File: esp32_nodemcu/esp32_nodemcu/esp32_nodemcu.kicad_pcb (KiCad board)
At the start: 2 copper layers, 17.8 x 30.5 mm, 3 parts, among them J1 Conn_01x02_Female

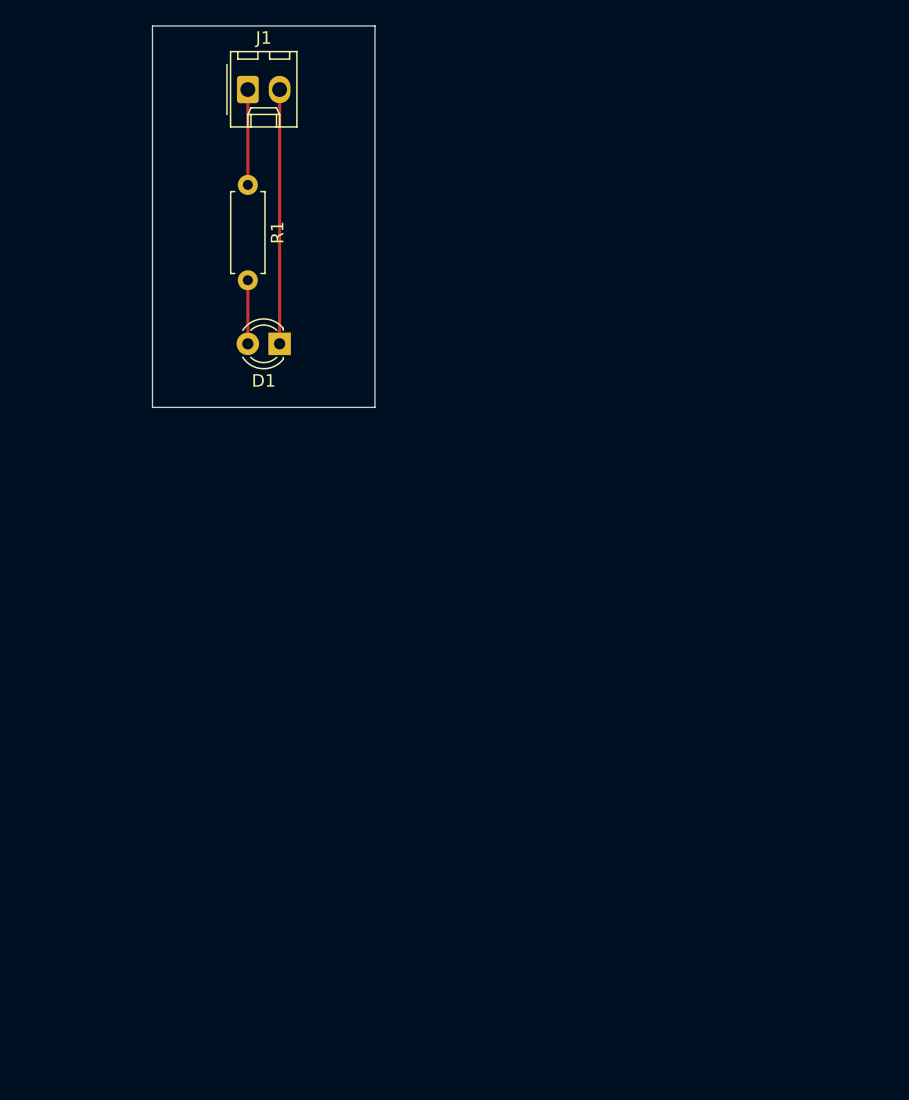
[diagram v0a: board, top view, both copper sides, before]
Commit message: pcb update
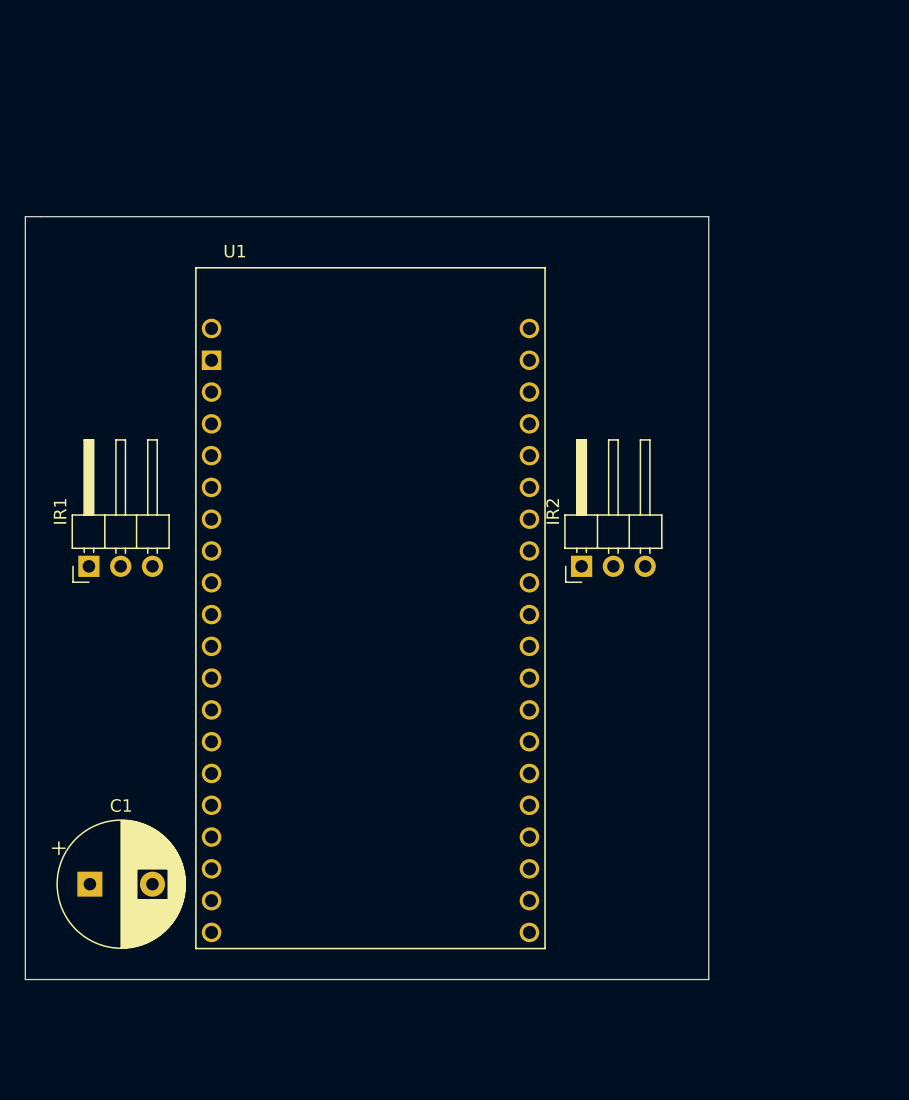
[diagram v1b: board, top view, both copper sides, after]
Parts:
- removed D1: LED, LED_THT:LED_D3.0mm
- removed J1: Conn_01x02_Female, Connector_Molex:Molex_KK-254_AE-6410-02A_1x02_P2.54mm_Vertical
- removed R1: R, Resistor_THT:R_Axial_DIN0207_L6.3mm_D2.5mm_P7.62mm_Horizontal
- added C1: CAP, Capacitor_THT:CP_Radial_D10.0mm_P5.00mm, F.Cu at (127.1, 124.5)
- added IR1: szh-ssbh-002, Connector_PinHeader_2.54mm:PinHeader_1x03_P2.54mm_Horizontal, F.Cu at (127.0, 99.1)
- added IR2: szh-ssbh-002, Connector_PinHeader_2.54mm:PinHeader_1x03_P2.54mm_Horizontal, F.Cu at (166.4, 99.1)
- added U1: ESP32-DEVKITC-32D, ESP32-DEVKITC-32D:MODULE_ESP32-DEVKITC-32D, F.Cu at (149.5, 102.4)
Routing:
- net GND: track 20.3 -> 0.00 mm
- net +5V: track 7.62 -> 0.00 mm
- net Net-(D1-Pad2): track 5.08 -> 0.00 mm
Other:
- board size 17.8 x 30.5 mm -> 54.6 x 61 mm

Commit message: pcb update
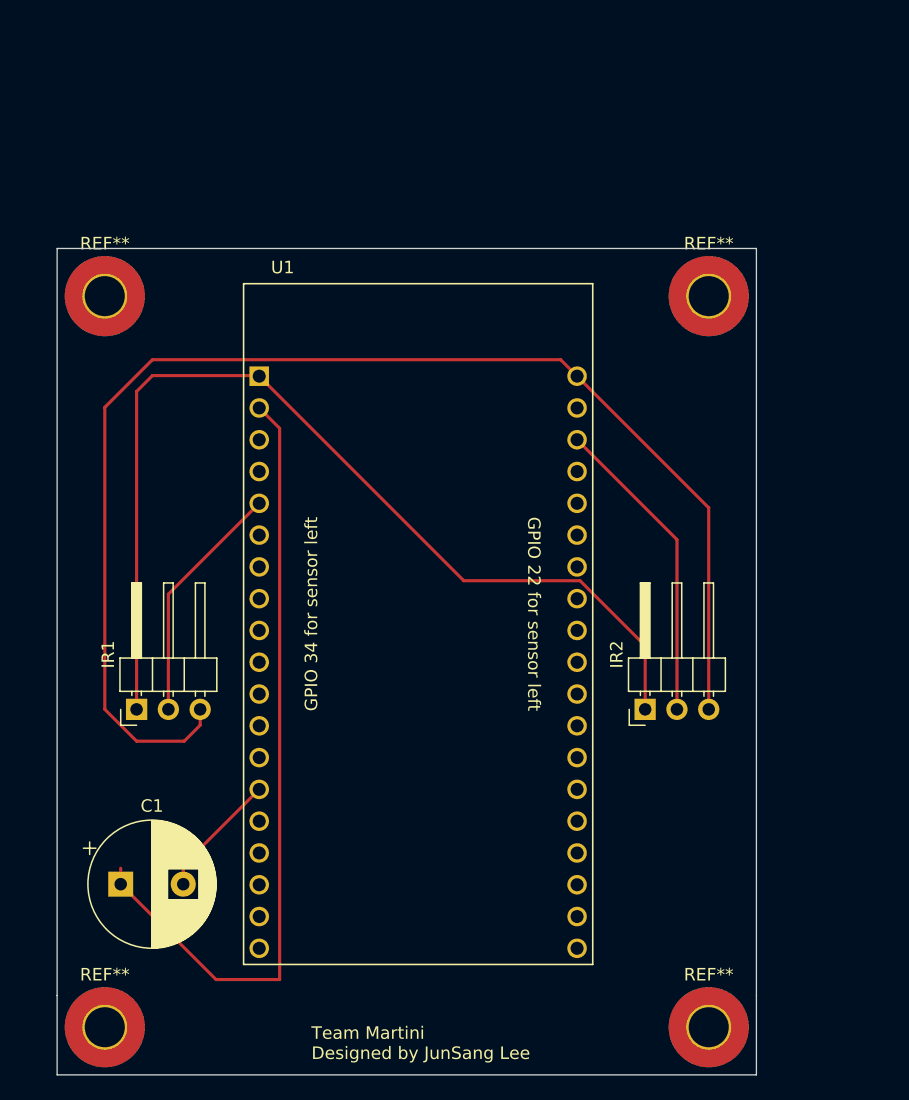
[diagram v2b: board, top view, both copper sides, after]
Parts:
- added REF**: MountingHole_3.2mm_M3_Pad_TopBottom, MountingHole:MountingHole_3.2mm_M3_Pad_TopBottom, F.Cu at (128.3, 135.9)
- added REF**: MountingHole_3.2mm_M3_Pad_TopBottom, MountingHole:MountingHole_3.2mm_M3_Pad_TopBottom, F.Cu at (176.5, 135.9)
- added REF**: MountingHole_3.2mm_M3_Pad_TopBottom, MountingHole:MountingHole_3.2mm_M3_Pad_TopBottom, F.Cu at (128.3, 77.5)
- added REF**: MountingHole_3.2mm_M3_Pad_TopBottom, MountingHole:MountingHole_3.2mm_M3_Pad_TopBottom, F.Cu at (176.5, 77.5)
- moved IR2 12.5 mm to (171.4, 110.5)
- moved IR1 12.0 mm to (130.8, 110.5)
- moved U1 4.02 mm to (153.3, 103.6)
- moved C1 2.46 mm to (129.5, 124.5)
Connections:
- U1 pad 15: Net-(IR2-Pad2) -> Net-(U1-Pad15)
- U1 pad 22: Net-(U1-Pad22) -> Net-(IR2-Pad2)
- U1 pad 3: Net-(IR1-Pad2) -> Net-(U1-Pad3)
- U1 pad 5: Net-(U1-Pad5) -> Net-(IR1-Pad2)
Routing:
- net Net-(IR1-Pad3): track 0.00 -> 105.4 mm
- net Net-(IR1-Pad1): track 0.00 -> 80.6 mm
- net Net-(C1-Pad1): track 0.00 -> 63.5 mm
- net Net-(IR2-Pad2): track 0.00 -> 24.9 mm
- net Net-(IR1-Pad2): track 0.00 -> 19.5 mm
- net Net-(C1-Pad2): track 0.00 -> 10.1 mm
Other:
- board size 54.6 x 61 mm -> 55.9 x 66 mm
- board text added: "GPIO 22 for sensor left"
- board text added: "GPIO 34 for sensor left"
- board text added: "Team Martini Designed by JunSang Lee"

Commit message: update pcb
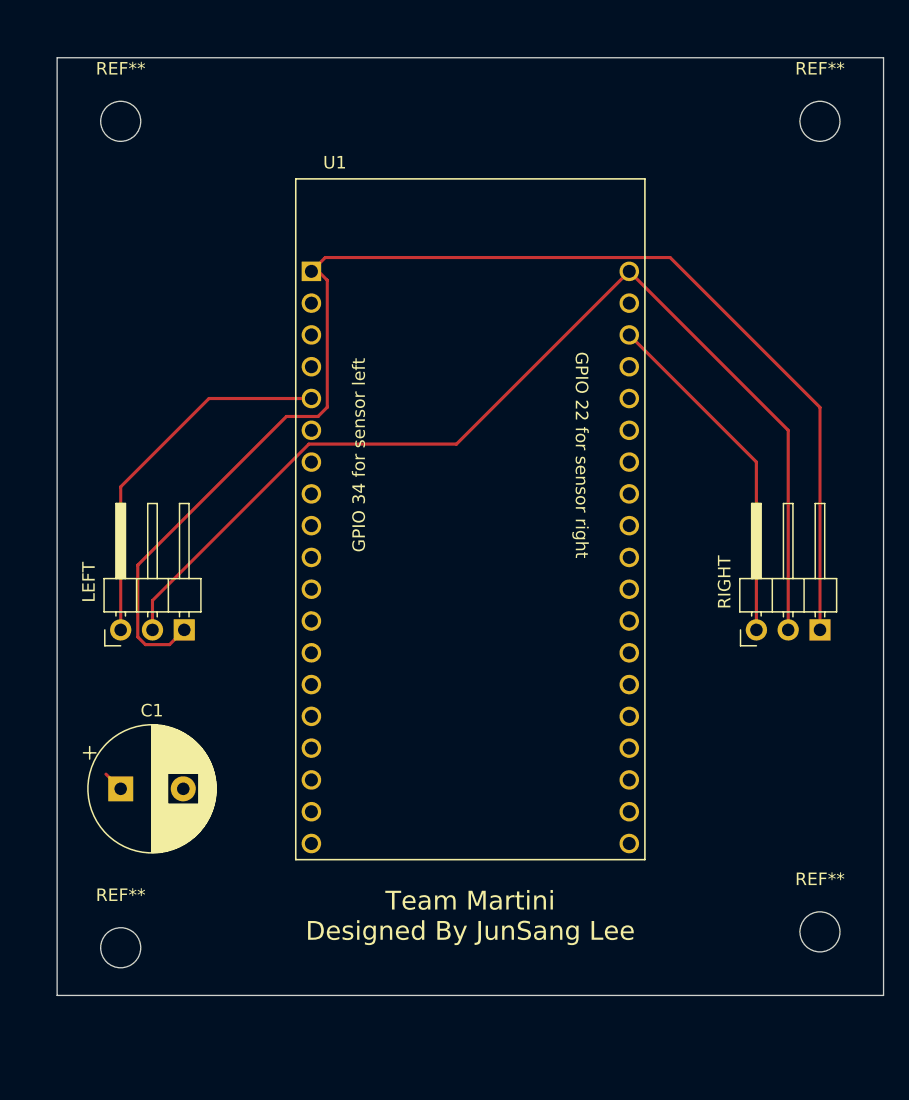
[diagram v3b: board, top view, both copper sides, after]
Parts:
- removed IR1, IR2: szh-ssbh-002, Connector_PinHeader_2.54mm:PinHeader_1x03_P2.54mm_Horizontal
- removed the REF** at (128.3, 135.9)
- removed the REF** at (176.5, 135.9)
- removed the REF** at (128.3, 77.5)
- removed the REF** at (176.5, 77.5)
- added LEFT: szh-ssbh-002, SZH-SSBH-002:szh-ssbh-002, F.Cu at (125.7, 100.3)
- added REF**: MountingHole_3.2mm_M3, MountingHole:MountingHole_3.2mm_M3, F.Cu at (129.5, 129.5)
- added REF**: MountingHole_3.2mm_M3, MountingHole:MountingHole_3.2mm_M3, F.Cu at (185.4, 128.3)
- added REF**: MountingHole_3.2mm_M3, MountingHole:MountingHole_3.2mm_M3, F.Cu at (129.5, 63.5)
- added REF**: MountingHole_3.2mm_M3, MountingHole:MountingHole_3.2mm_M3, F.Cu at (185.4, 63.5)
- added RIGHT: szh-ssbh-002, SZH-SSBH-002:szh-ssbh-002, F.Cu at (176.5, 100.3)
- moved U1 9.36 mm to (157.5, 95.2)
- moved C1 7.62 mm to (129.5, 116.8)
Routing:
- net Net-(C1-Pad1): track 63.5 -> 1.66 mm
- net Net-(IR1-Pad1): track 80.6 -> 106.1 mm
- net Net-(IR1-Pad2): track 105.4 -> 85.3 mm
- net Net-(IR1-Pad3): track 19.5 -> 29.6 mm
- net Net-(C1-Pad2): track 10.1 -> 0.00 mm
- net Net-(IR2-Pad3): track 24.9 -> 27.8 mm
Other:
- board size 55.9 x 66 mm -> 66 x 74.9 mm
- board text added: "GPIO 22 for sensor right"
- board text added: "Team Martini Designed By JunSang Lee"
- board text removed: "GPIO 22 for sensor left"
- board text removed: "Team Martini Designed by JunSang Lee"
